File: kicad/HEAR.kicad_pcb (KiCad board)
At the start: 2 copper layers, 39.3 x 106.5 mm, 56 parts, among them J1 PJ341, J12 Euro power header, J13 PJ341, J14 PJ341, J2 PJ341, J3 PJ341, J4 PJ341, J5 Attenuator Jumper 1, J6 Attenuator Jumper 2, U1 TL074, U2 RC4580

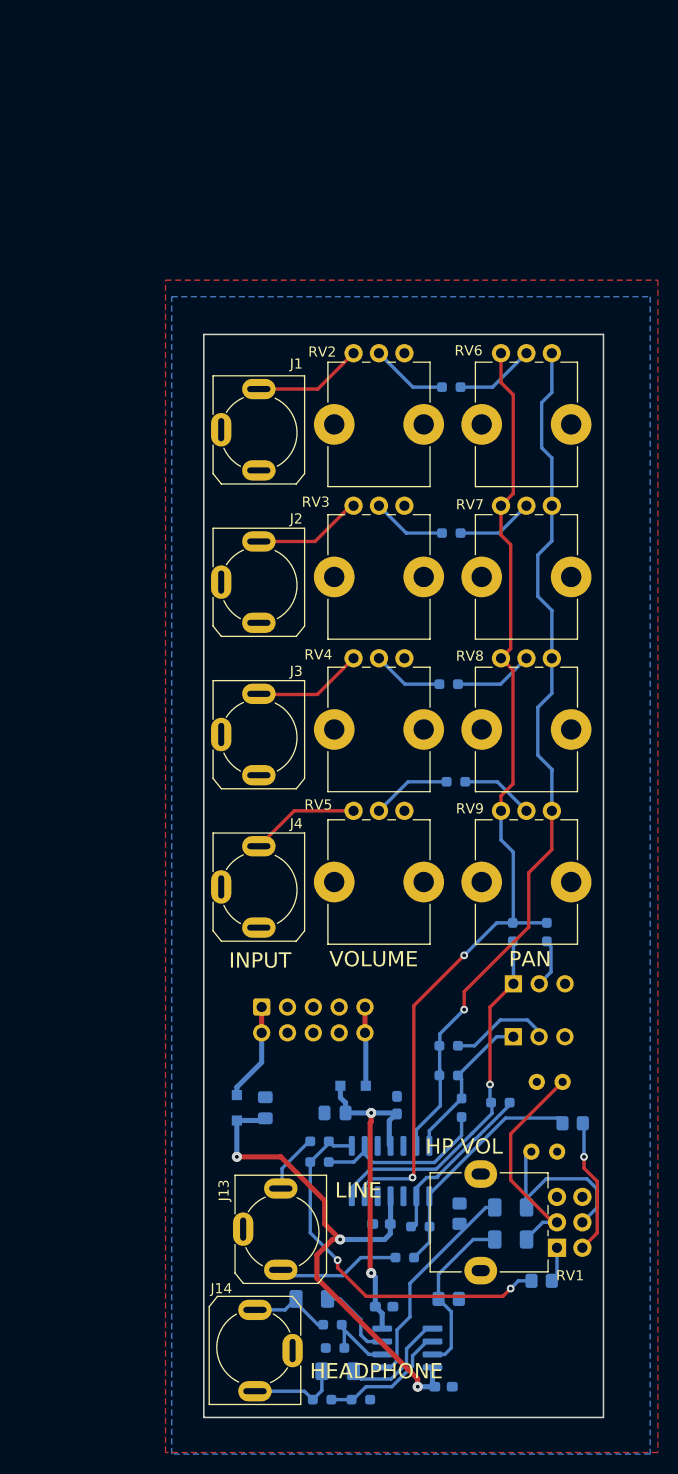
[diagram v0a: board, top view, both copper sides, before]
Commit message: footprints submodule
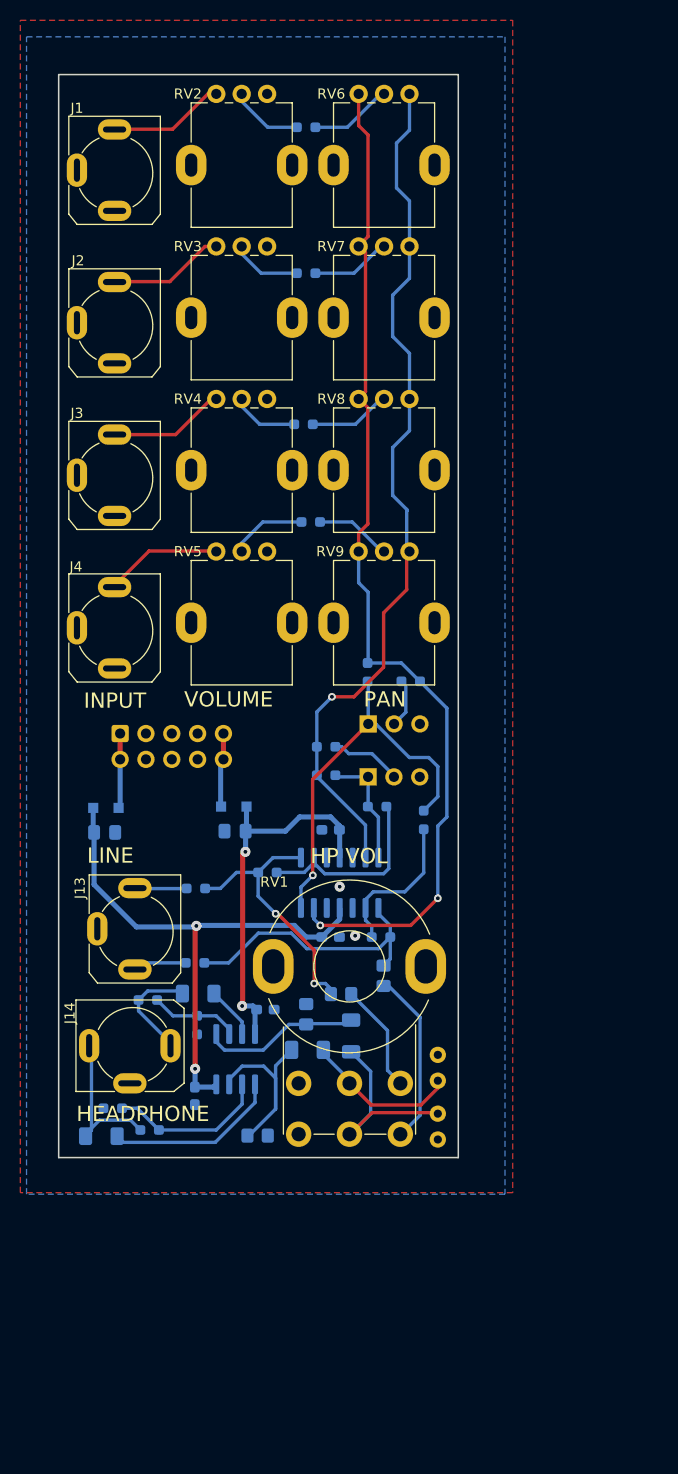
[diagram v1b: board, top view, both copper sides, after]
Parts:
- J1, J13, J14, J2, J3, J4: footprint nearness:PJ341 -> Crows:PJ341
- RV1: footprint Potentiometer_THT:Potentiometer_Alpha_RD902F-40-00D_Dual_Vertical -> Crows:RV1666G-F
- RV2, RV3, RV4, RV5, RV6, RV7, RV8, RV9: footprint Potentiometer_THT:Potentiometer_Alps_RK09K_Single_Vertical -> Crows:RotaryPotVerticalSingle9mm
- moved R23 37.6 mm to (5.31, 101.6), turned to 0 degrees
- moved C10 37.6 mm to (13.4, 100.4), turned to 90 degrees
- moved R26 36.7 mm to (8.77, 91.0)
- moved R30 35.6 mm to (13.4, 87.4)
- moved R24 34.5 mm to (13.6, 93.5), turned to 90 degrees
- moved R35 34.4 mm to (27.8, 90.4)
- moved RV1 34.4 mm to (28.6, 87.7), turned to 0 degrees
- moved U2 33.0 mm to (17.4, 96.8), turned to 90 degrees
- moved J13 32.8 mm to (7.50, 84.0)
- moved R33 32.8 mm to (4.20, 104.4)
- moved J14 32.4 mm to (7.00, 95.5), turned to -90 degrees
- moved D2 32.2 mm to (4.65, 72.1), turned to 180 degrees
- moved R34 32.0 mm to (13.7, 90.4)
- moved R17 31.9 mm to (26.3, 68.9)
- moved R38 31.8 mm to (26.3, 66.1)
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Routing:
- net Lout: track 37.6 -> 26.4 mm
- net Net-(R35-Pad1): track 3.46 -> 10.8 mm
- net RLineOut: track 12.3 -> 5.27 mm
- net HPoutL: track 9.19 -> 15.8 mm
- net Net-(C1-Pad1): track 21.8 -> 15.3 mm
- net Net-(R33-Pad2): track 11.0 -> 17.2 mm
- net Net-(C2-Pad2): track 21.4 -> 15.6 mm
- net +12V: track 33.3 -> 37.1 mm
- net Net-(R36-Pad1): track 13.4 -> 17.2 mm, vias 1 -> 0
- net Rout: track 23.3 -> 27.0 mm
- net Net-(J5-Pad1): track 15.4 -> 11.7 mm
- net /RightMix: track 98.8 -> 101.8 mm
- net Net-(J5-Pad2): track 10.1 -> 7.06 mm
- net Net-(J6-Pad1): track 35.6 -> 38.5 mm
- net Net-(R34-Pad2): track 8.00 -> 5.12 mm
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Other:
- board text added: "RED"
